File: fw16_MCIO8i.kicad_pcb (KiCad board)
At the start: 6 copper layers, 105.4 x 94.3 mm, 21 parts, among them U1 SY75602ATWL-TR

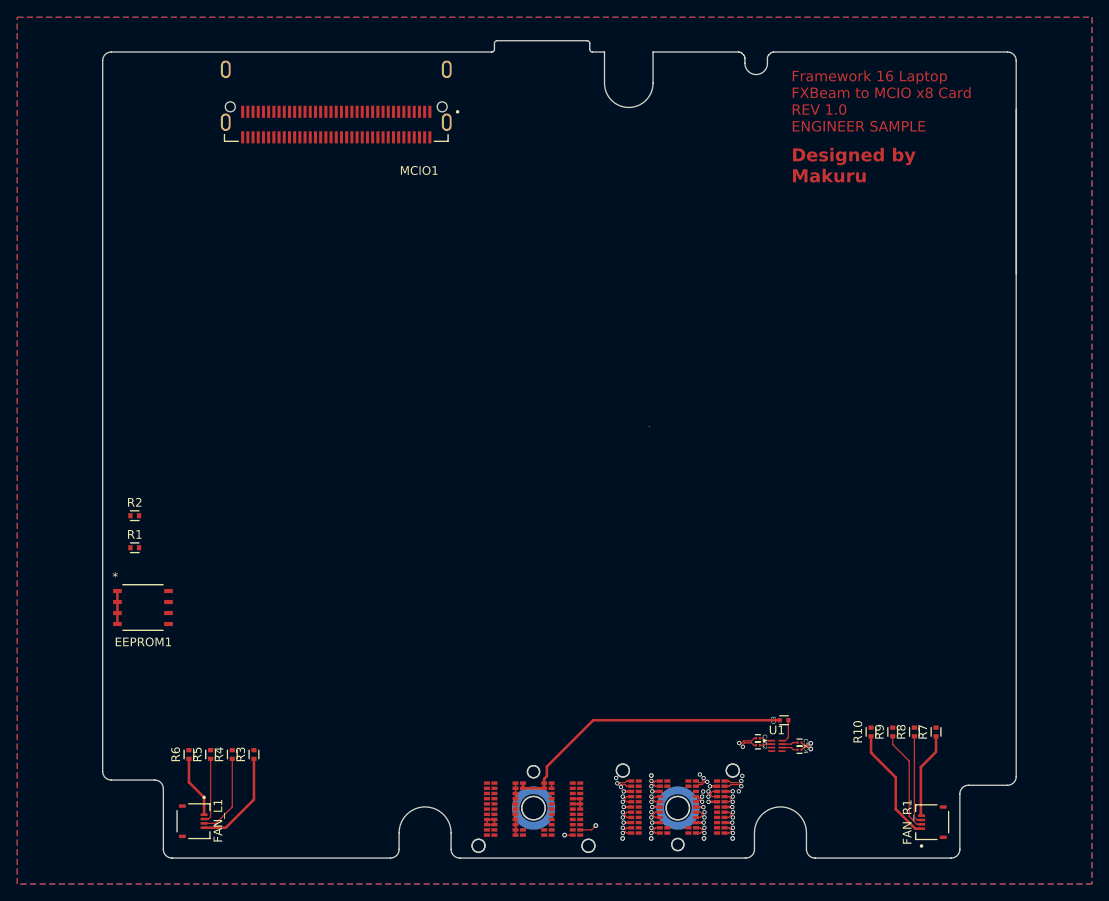
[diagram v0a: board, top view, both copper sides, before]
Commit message: Routing
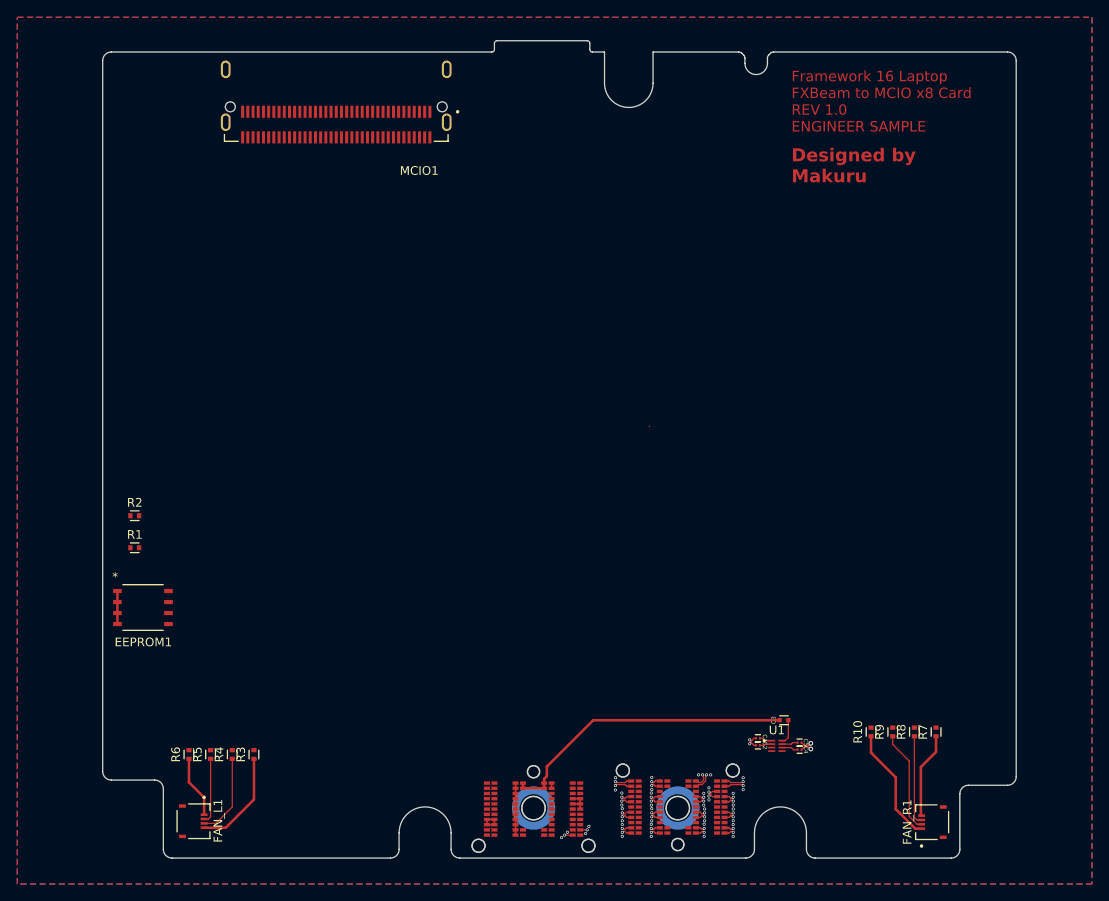
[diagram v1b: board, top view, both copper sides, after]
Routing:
- net /MCIO/PCI.TX5+: track 41.6 -> 13.9 mm
- net /MCIO/PCI.TX5-: track 41.0 -> 13.7 mm
- net GND: track 28.0 -> 16.3 mm, vias 23 -> 38
- net /MCIO/PCI.TX3-: track 16.9 -> 26.3 mm
- net /MCIO/PCI.TX3+: track 17.4 -> 26.8 mm
- net /MCIO/PCI.TX4-: track 13.4 -> 20.3 mm
- net /MCIO/PCI.TX4+: track 13.2 -> 19.8 mm
- net /MCIO/PCI.RX7+: track 10.7 -> 5.58 mm
- net /MCIO/PCI.TX0+: track 24.1 -> 19.0 mm
- net /MCIO/PCI.TX0-: track 23.5 -> 18.4 mm
- net /MCIO/PCI.RX7-: track 10.4 -> 5.41 mm
- net /MCIO/PCI.TX1+: track 25.3 -> 20.9 mm
- net /MCIO/PCI.TX1-: track 24.7 -> 20.3 mm
- net /MCIO/PCI.RX4-: track 11.2 -> 7.95 mm
- net /MCIO/PCI.RX4+: track 10.9 -> 7.74 mm
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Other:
- outline, holes or cut-outs redrawn
